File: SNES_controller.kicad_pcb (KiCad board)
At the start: 2 copper layers, 144 x 62 mm, 23 parts, among them J1 Conn_01x07, SW1 R, SW10 SELECT, SW11 Y, SW12 B, SW2 L, SW3 X, SW4 A, SW5 RIGHT, SW6 LEFT, SW7 DOWN, SW8 UP, SW9 START, U1 4021, U2 4021, U3 4069, U4 4011

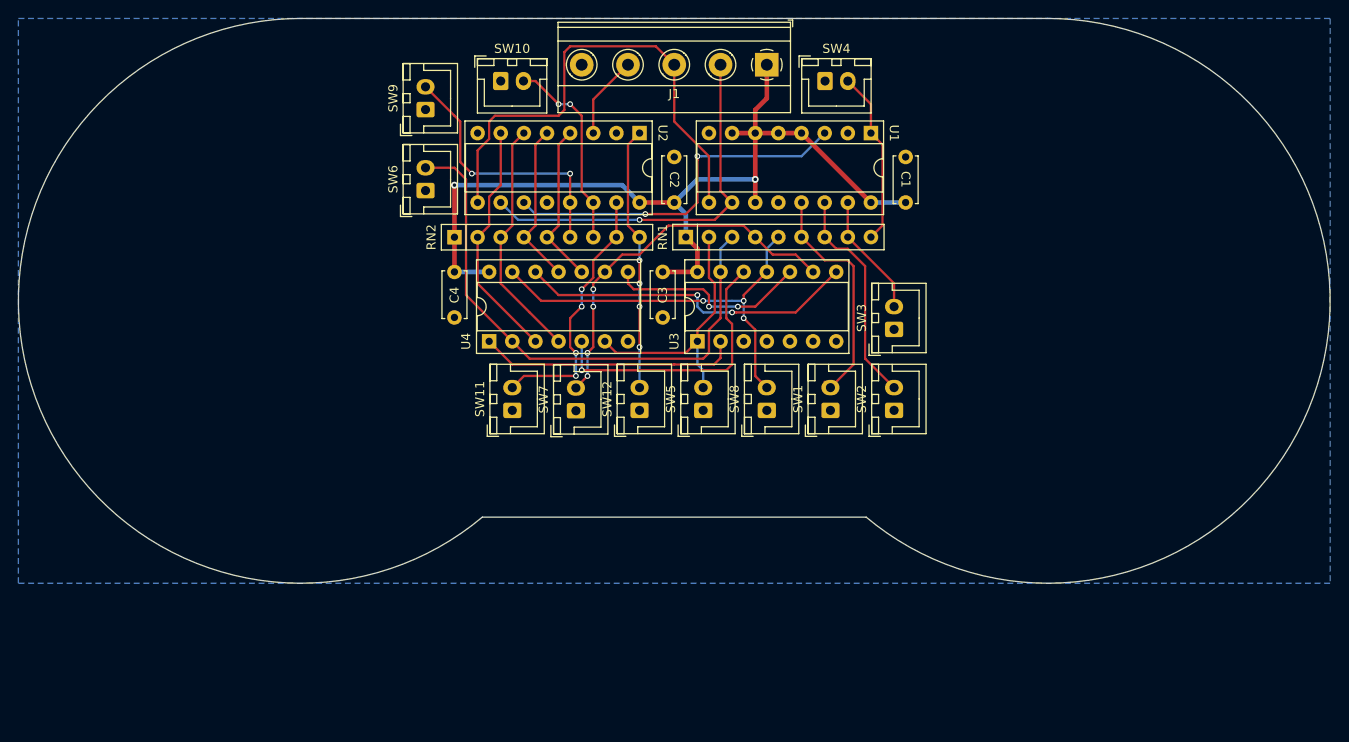
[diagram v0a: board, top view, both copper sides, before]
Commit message: Finish redesign
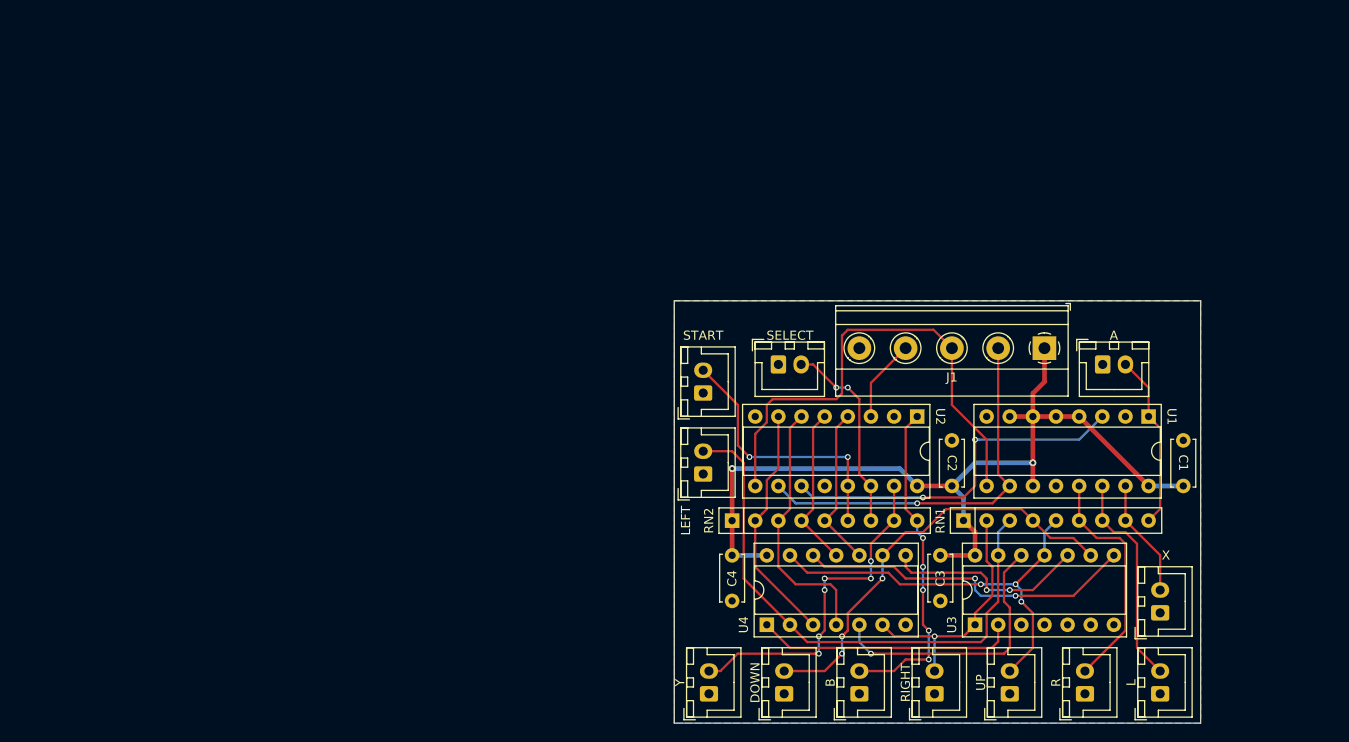
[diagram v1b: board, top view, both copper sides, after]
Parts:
- moved C1 43.6 mm to (55.9, 20.3)
- moved U3 43.6 mm to (33.0, 35.6)
- moved C2 43.6 mm to (30.5, 20.3)
- moved C3 43.6 mm to (29.2, 27.9)
- moved C4 43.6 mm to (6.35, 27.9)
- moved J1 43.6 mm to (40.6, 5.20)
- moved RN1 43.6 mm to (31.8, 24.1)
- moved SW10 43.6 mm to (11.4, 6.99)
- moved SW4 43.6 mm to (47.0, 6.99)
- moved SW6 43.6 mm to (3.17, 19.0)
- moved SW9 43.6 mm to (3.17, 10.1)
- moved U1 43.6 mm to (52.1, 12.7)
- moved U2 43.6 mm to (26.7, 12.7)
- moved U4 43.6 mm to (10.2, 35.6)
- moved RN2 43.6 mm to (6.35, 24.1)
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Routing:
- net Net-(RN2-Pad8): track 28.9 -> 37.7 mm, vias 4 -> 6
- net Net-(RN2-Pad9): track 29.0 -> 36.4 mm, vias 4 -> 5
- net Net-(RN1-Pad4): track 41.2 -> 46.8 mm, vias 4 -> 3
- net /LEFT: track 26.5 -> 28.8 mm
- net Net-(RN1-Pad2): track 29.1 -> 27.5 mm, vias 0 -> 1
- net Net-(U3-Pad12): track 31.2 -> 30.4 mm
- net Net-(RN1-Pad7): track 24.2 -> 23.7 mm
- net Net-(RN1-Pad8): track 13.5 -> 13.0 mm
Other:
- board size 144 x 62 mm -> 57.8 x 46.4 mm
